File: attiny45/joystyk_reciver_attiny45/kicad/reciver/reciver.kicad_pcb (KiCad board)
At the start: 2 copper layers, 14 parts, among them J1 DRIVES, J2 XY-MK-5V, J3 PWR, U1 ATtiny45-20PU, U2 L7805, U3 LM317_3PinPackage

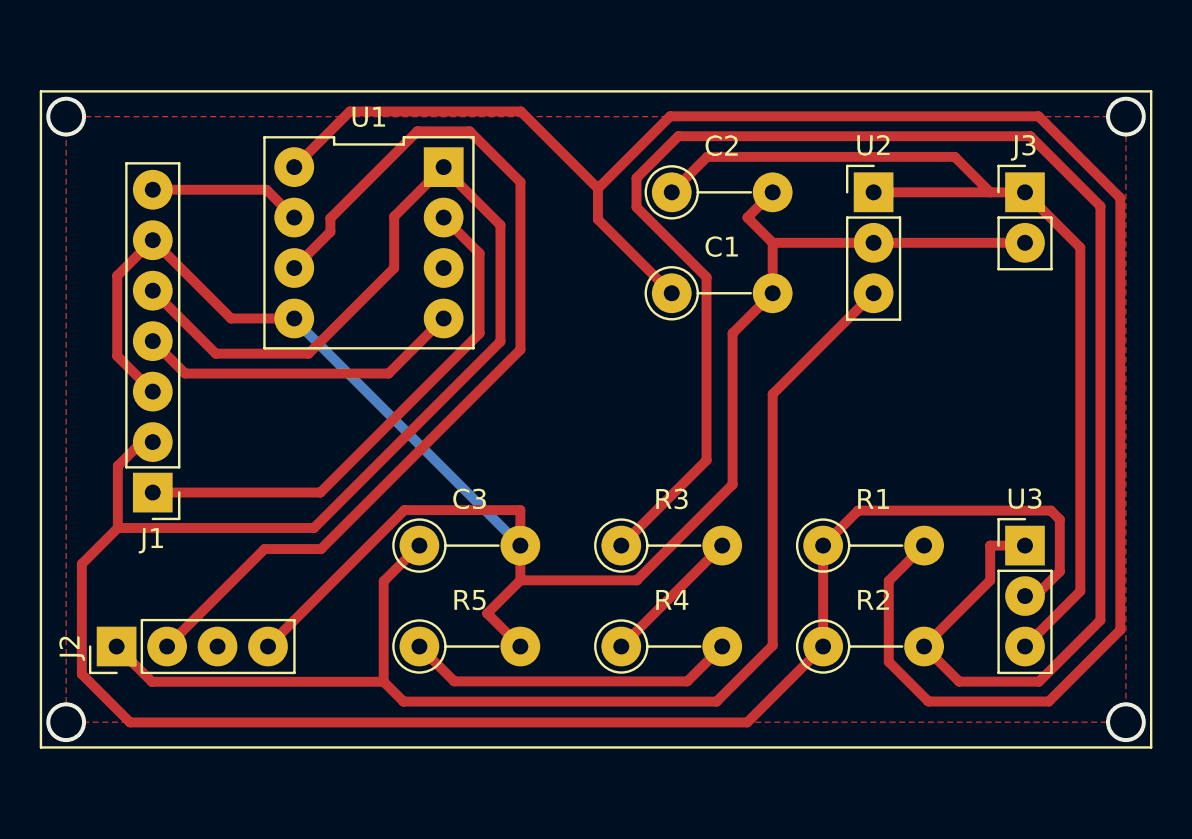
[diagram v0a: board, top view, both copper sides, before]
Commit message: Added renew recv kicad scheme
Signed-off-by: Alexey B <bayrepo.info@gmail.com>
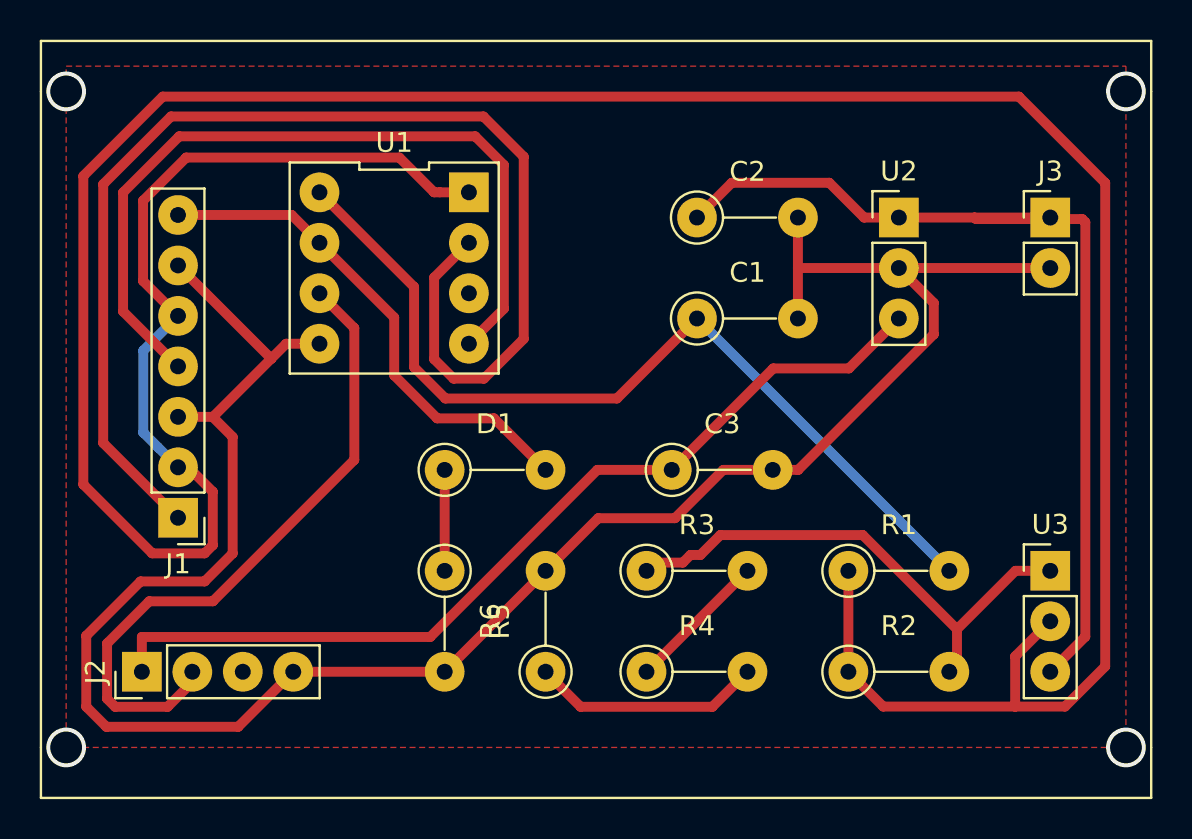
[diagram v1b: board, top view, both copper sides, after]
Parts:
- added D1: LED, transmitter:R_my_5_08, F.Cu at (121.9, 92.7)
- added R6: 220, transmitter:R_my_5_08, F.Cu at (121.9, 97.8)
- moved C3 13.3 mm to (133.3, 92.7)
- moved R5 6.48 mm to (127.0, 102.9), turned to 90 degrees
- moved C1 1.80 mm to (134.6, 85.1)
- moved C2 1.80 mm to (134.6, 80.0)
- moved J2 1.80 mm to (106.7, 102.9)
- moved J3 1.80 mm to (152.4, 80.0)
- moved R1 1.80 mm to (142.2, 97.8)
- moved R2 1.80 mm to (142.2, 102.9)
- moved R3 1.80 mm to (132.1, 97.8)
- moved R4 1.80 mm to (132.1, 102.9)
- moved U2 1.80 mm to (144.8, 80.0)
- moved U3 1.80 mm to (152.4, 97.8)
- moved J1 1.80 mm to (108.5, 95.1)
- moved U1 1.80 mm to (119.4, 82.5)
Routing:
- net Net-(R2-Pad2): track 87.4 -> 26.5 mm
- net Net-(C1-Pad1): track 96.7 -> 45.3 mm
- net Net-(J1-Pad1): track 26.3 -> 63.3 mm
- net Net-(J1-Pad2): track 130.6 -> 166.0 mm
- net Net-(J1-Pad4): track 16.5 -> 40.6 mm
- net Net-(D1-Pad2): track 7.70 -> 25.5 mm
- net Net-(C3-Pad1): track 62.8 -> 46.5 mm
- net Net-(J2-Pad2): track 48.1 -> 33.7 mm
- net GND: track 99.8 -> 108.3 mm
- net Net-(D1-Pad1): track 0.00 -> 5.08 mm
- net Net-(R4-Pad2): track 16.7 -> 11.6 mm
- net VCC: track 50.3 -> 48.3 mm
